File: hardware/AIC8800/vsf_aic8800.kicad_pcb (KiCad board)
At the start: 2 copper layers, 27.9 x 52.1 mm, 31 parts, among them J0 USB_C_Receptacle_USB2.0, J1 Conn_01x20, J2 Conn_01x20, J3 Conn_02x05_Counter_Clockwise, Q0 AO3401, Q1 AO3402, SW0 SW_Push, SW1 SW_Push, U0 Module_AIC8800M

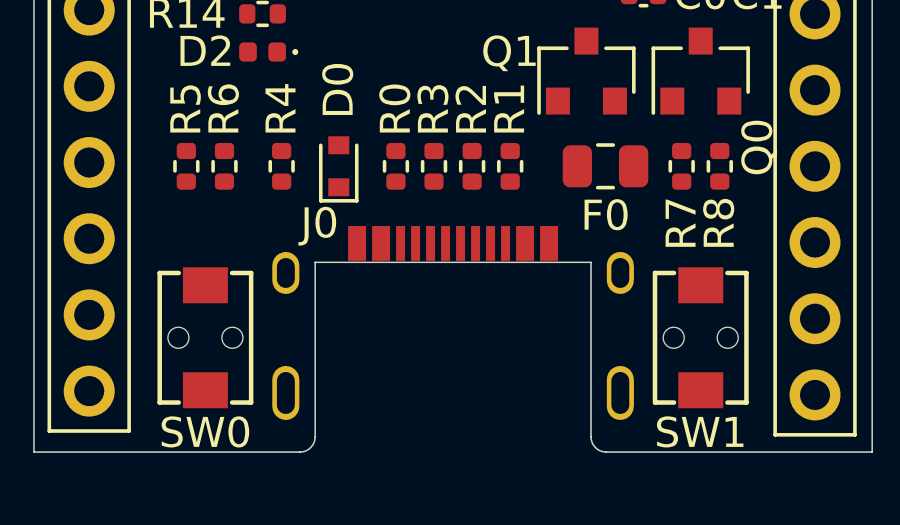
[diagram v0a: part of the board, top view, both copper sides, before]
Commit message: [hardware/aic8800] minor tweak
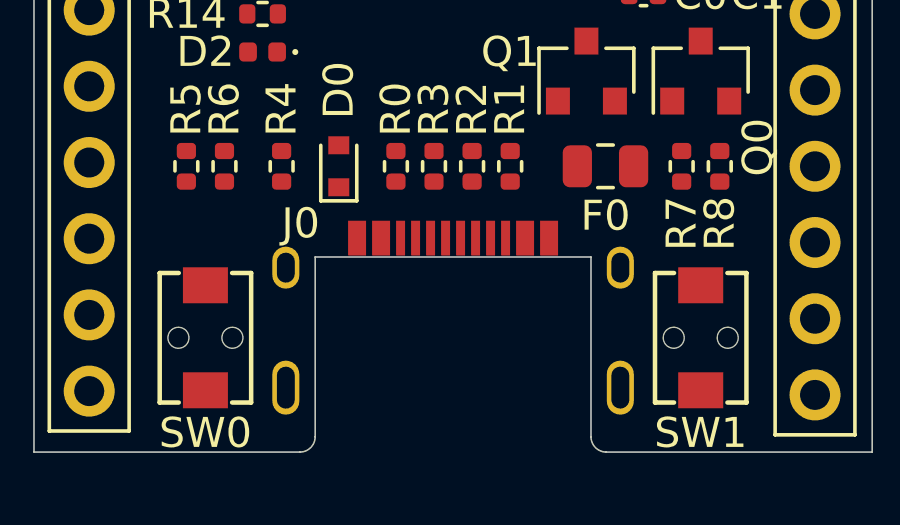
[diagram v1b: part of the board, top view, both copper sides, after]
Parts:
- moved J0 0.18 mm to (217.2, 149.0)
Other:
- outline, holes or cut-outs redrawn
